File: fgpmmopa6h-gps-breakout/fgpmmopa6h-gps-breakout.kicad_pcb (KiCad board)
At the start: 2 copper layers, 43.2 x 28 mm, 15 parts, among them J1 BREAKOUT, U1 MIC5365, U2 FGPMMOPA6H-GPS

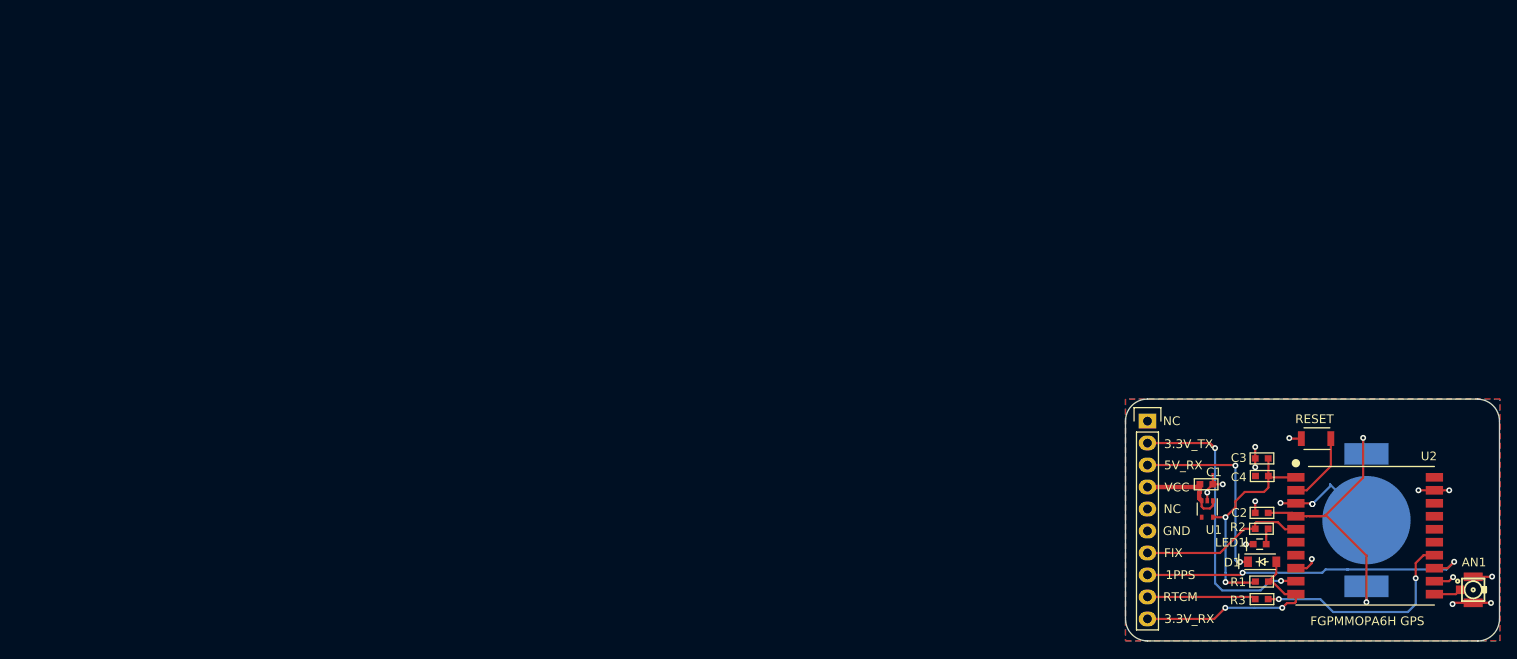
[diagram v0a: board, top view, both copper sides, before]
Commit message: Regenerated bom and gerbers.
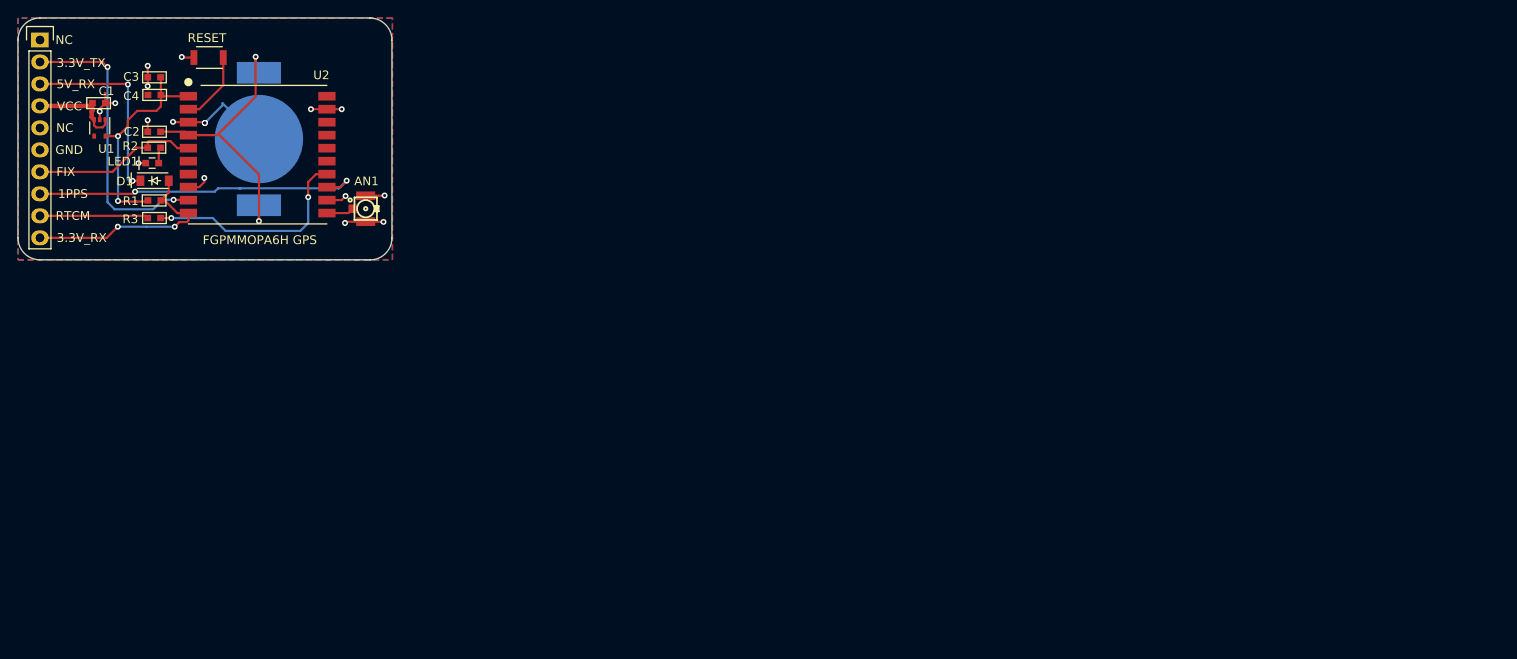
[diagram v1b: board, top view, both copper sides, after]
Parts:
- moved AN1 135.3 mm to (40.5, 56.7)
- moved BAT1 135.3 mm to (28.2, 48.7)
- moved D1 135.3 mm to (16.1, 53.5)
- moved LED1 135.3 mm to (15.8, 51.5)
- moved S1 135.3 mm to (24.0, 39.3)
- moved U2 135.3 mm to (28.0, 50.5)
- moved C1 135.3 mm to (9.67, 44.6)
- moved C2 135.3 mm to (16.1, 47.9)
- moved C3 135.3 mm to (16.1, 41.6)
- moved C4 135.3 mm to (16.1, 43.6)
- moved J1 135.3 mm to (2.87, 37.3)
- moved R1 135.3 mm to (16.1, 55.8)
- moved R2 135.3 mm to (16.1, 49.7)
- moved R3 135.3 mm to (16.1, 57.8)
- moved U1 135.3 mm to (9.77, 47.4)
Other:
- board text added: "FABRICATION NOTES 1. THIS IS A 2 LAYER BOARD. 2. EXTERNAL LAYERS SHALL HAVE 1 OZ COPPER. 3. MATERIAL: FR4 AND 0.062 INCH +/- 10% THICK. 4. BOARDS SHALL BE ROHS COMPLIANT. 5. MANUFACTURE IN ACCORDANCE WITH IPC-6012 CLASS 2 6. MASK: BOTH SIDES OF THE BOARD SHALL HAVE SOLDER MASK (ANY COLOR) OVER BARE COPPER. 7. SILK: BOTH SIDES OF THE BOARD SHALL HAVE WHITE SILKSCREEN. DO NOT PLACE SILK OVER BARE C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"
